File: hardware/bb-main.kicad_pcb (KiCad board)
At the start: 2 copper layers, 29.8 x 25.4 mm, 27 parts, among them P1 USB_B, P2 PICkit3, P3 OLED, SW1 SW_PUSH, U1 BU33TD3WG-TR, U2 PIC16(L)F1455-I/SL

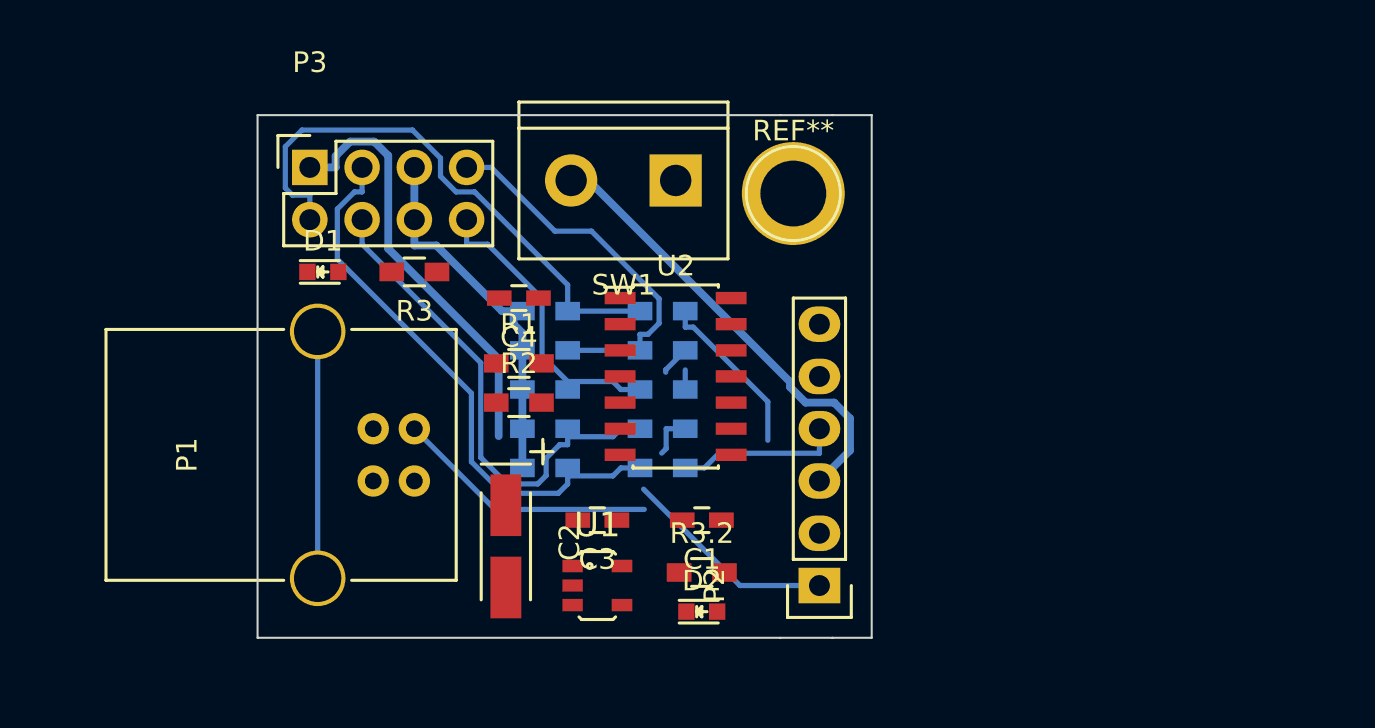
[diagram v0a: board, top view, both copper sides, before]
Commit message: Board changes
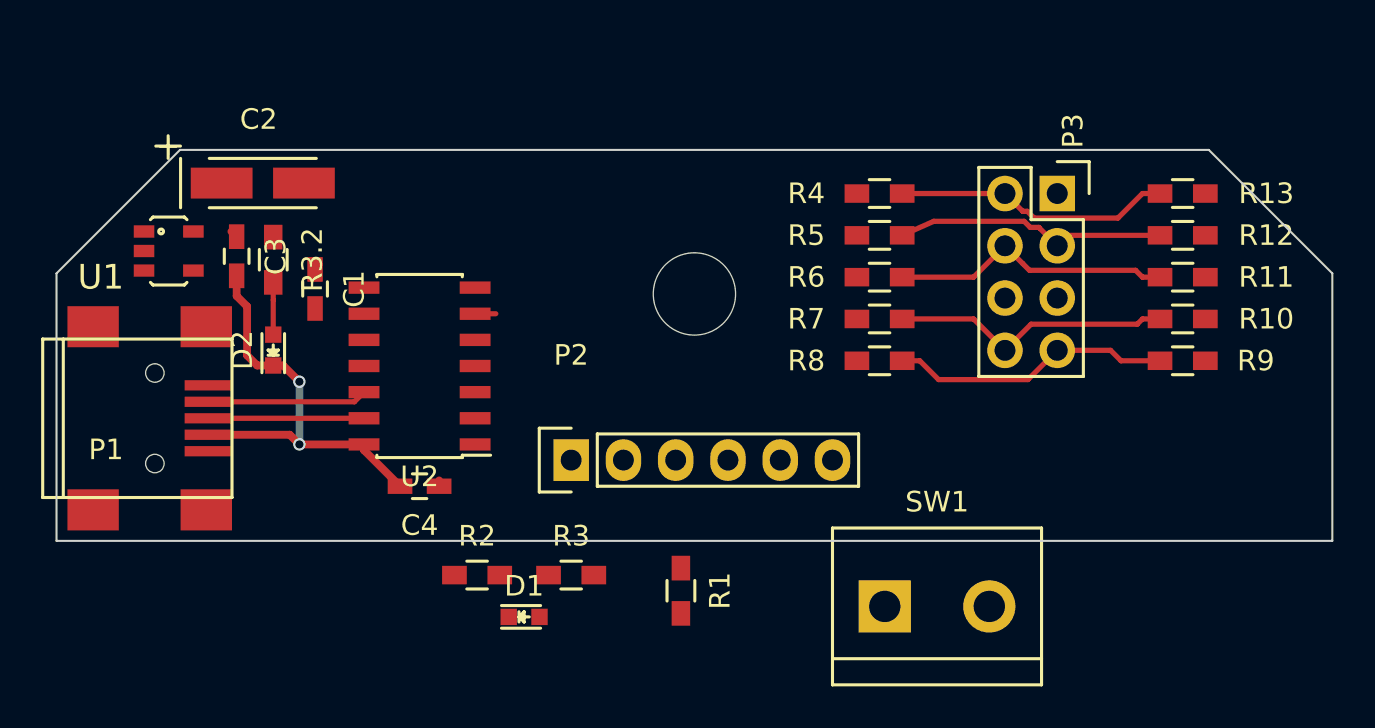
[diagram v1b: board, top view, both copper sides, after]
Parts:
- removed REF**: 1pin, Connect:1pin
- added MH1: , Mounting_Holes:MountingHole_4mm, F.Cu at (86.0, 76.0)
- D2: value Led_Small -> L1
- P1: footprint Connect:USB_B -> Connect:USB_Mini-B
- R10, R11, R12, R13, R4, R5, R6, R7, R8, R9: moved to F.Cu
- moved P3 36.3 mm to (103.6, 71.1), turned to 270 degrees
- moved R12 33.0 mm to (109.7, 73.2), turned to 180 degrees
- moved R11 31.9 mm to (109.7, 75.2), turned to 180 degrees
- moved R13 31.5 mm to (109.7, 71.1), turned to 180 degrees
- moved R10 31.2 mm to (109.7, 77.2), turned to 180 degrees
- moved R9 31.0 mm to (109.7, 79.2), turned to 180 degrees
- moved U1 26.4 mm to (60.5, 73.9)
- moved R3.2 25.8 mm to (65.5, 74.3), turned to 270 degrees
- moved SW1 25.7 mm to (97.8, 91.2), turned to 0 degrees
- moved D2 24.4 mm to (65.5, 78.7), turned to 90 degrees
- moved C1 21.9 mm to (67.6, 75.8), turned to 270 degrees
- moved C3 21.7 mm to (63.8, 74.2), turned to 270 degrees
- moved C2 21.2 mm to (65.0, 70.6), turned to 0 degrees
- moved D1 19.4 mm to (77.7, 91.7)
- moved R3 16.6 mm to (80.0, 89.7), turned to 0 degrees
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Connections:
- P2 pad 6: (no net) -> Net-(P2-Pad6)
- U1 pad 4: (no net) -> Net-(U1-Pad4)
- U2 pad 2: /LED_A -> /BUT_1
- U2 pad 3: /BUT_1 -> /LED_A
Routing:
- net +3V3: track 20.8 -> 0.39 mm
- net GND: track 40.3 -> 21.9 mm, vias 0 -> 2
- net /SCK: track 27.7 -> 13.5 mm
- net /SDO: track 27.0 -> 13.5 mm
- net Net-(P1-Pad5): track 12.0 -> 0.00 mm
- net /D/~C~: track 24.4 -> 13.8 mm
- net /~MCLR~: track 10.5 -> 1.92 mm
- net /OLED_SDO: track 8.17 -> 0.15 mm
- net Net-(P1-Pad3): track 0.00 -> 7.57 mm
- net /ICSPDAT/OLED_SCK: track 8.01 -> 0.45 mm
- net Net-(P1-Pad2): track 12.8 -> 7.76 mm
- net /~RES~: track 18.6 -> 13.7 mm
- net Net-(D2-Pad2): track 0.00 -> 2.54 mm
- net /OLED_D/~C~: track 2.20 -> 0.15 mm
- net /OLED_~RES~: track 1.46 -> 0.00 mm
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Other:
- board size 29.8 x 25.4 mm -> 62 x 19 mm

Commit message: Board rework
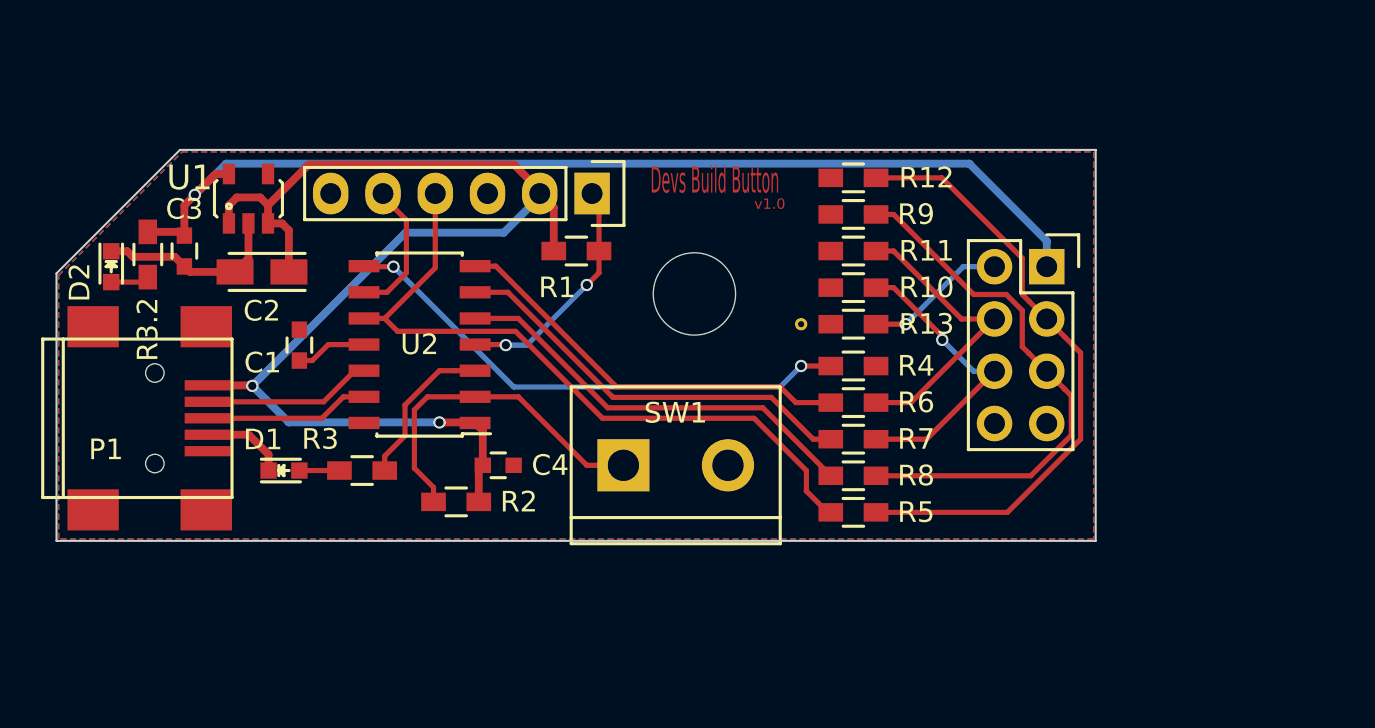
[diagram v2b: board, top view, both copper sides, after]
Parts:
- added ?: , Housings_Proj:VIA-0.6mm, F.Cu at (91.2, 77.5)
- C1, C3, C4: footprint Capacitors_SMD:C_0603_HandSoldering -> Capacitors_SMD:C_0603
- C2: footprint Capacitors_Tantalum_SMD:TantalC_SizeA_EIA-3216_HandSoldering -> Capacitors_Tantalum_SMD:TantalC_SizeA_EIA-3216_Reflow
- D2: value L1 -> Led_Small
- moved R9 17.5 mm to (93.7, 72.1), turned to 0 degrees
- moved R1 17.3 mm to (80.3, 73.9), turned to 0 degrees
- moved R13 17.2 mm to (93.7, 77.5), turned to 0 degrees
- moved R12 16.2 mm to (93.7, 70.4), turned to 0 degrees
- moved R10 16.1 mm to (93.7, 75.7), turned to 0 degrees
- moved R11 16.1 mm to (93.7, 73.9), turned to 0 degrees
- moved SW1 14.4 mm to (85.1, 84.3)
- moved D1 13.7 mm to (66.1, 84.6)
- moved R5 13.5 mm to (93.7, 86.6)
- moved P2 13.0 mm to (81.0, 71.1), turned to 180 degrees
- moved R3 11.4 mm to (69.8, 84.6), turned to 180 degrees
- moved D2 8.86 mm to (57.7, 74.7), turned to 270 degrees
- moved R4 8.48 mm to (93.7, 79.5)
- moved R6 6.23 mm to (93.7, 81.3)
- moved R3.2 6.10 mm to (59.4, 74.1)
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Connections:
- P1 pad 5: Net-(P1-Pad5) -> (no net)
- P2 pad 6: Net-(P2-Pad6) -> (no net)
- P3 pad 5: GND -> /~RES~
- P3 pad 6: GND -> /~CS~
- P3 pad 7: /~RES~ -> GND
- P3 pad 8: /~CS~ -> GND
- U1 pad 4: Net-(U1-Pad4) -> (no net)
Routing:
- net +5V: track 0.71 -> 60.8 mm, vias 0 -> 2
- net +3V3: track 0.39 -> 51.0 mm, vias 0 -> 1
- net /ICSPDAT/OLED_SCK: track 0.45 -> 34.3 mm
- net /OLED_SDO: track 0.15 -> 25.5 mm, vias 0 -> 2
- net /OLED_~RES~: track 0.00 -> 20.4 mm
- net /OLED_D/~C~: track 0.15 -> 20.0 mm
- net /OLED_~CS~: track 1.15 -> 20.2 mm
- net /BUT_1: track 0.00 -> 16.7 mm
- net /SCK: track 13.5 -> 30.1 mm
- net /~RES~: track 13.7 -> 26.4 mm
- net /~MCLR~: track 1.92 -> 11.6 mm, vias 0 -> 2
- net GND: track 21.9 -> 13.2 mm, vias 2 -> 0
- net /LED_A: track 0.00 -> 7.69 mm
- net /SDO: track 13.5 -> 6.92 mm, vias 0 -> 1
- net /ICSPCLK: track 0.60 -> 6.77 mm
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- added copper zone on B.Cu, net GND
- added copper zone on F.Cu, net GND
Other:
- board size 62 x 19 mm -> 50.5 x 19 mm
- board text added: "Devs Build Button"
- board text added: "v1.0"
